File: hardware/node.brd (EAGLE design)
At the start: 16.5 x 25.7 mm, 56 parts, among them IC1 MAX1555, Q1 P-MOSFET, U1 ATMEGA32U4, U2 MCP1703CB/TOREX-XC6206, Y1 8MHz

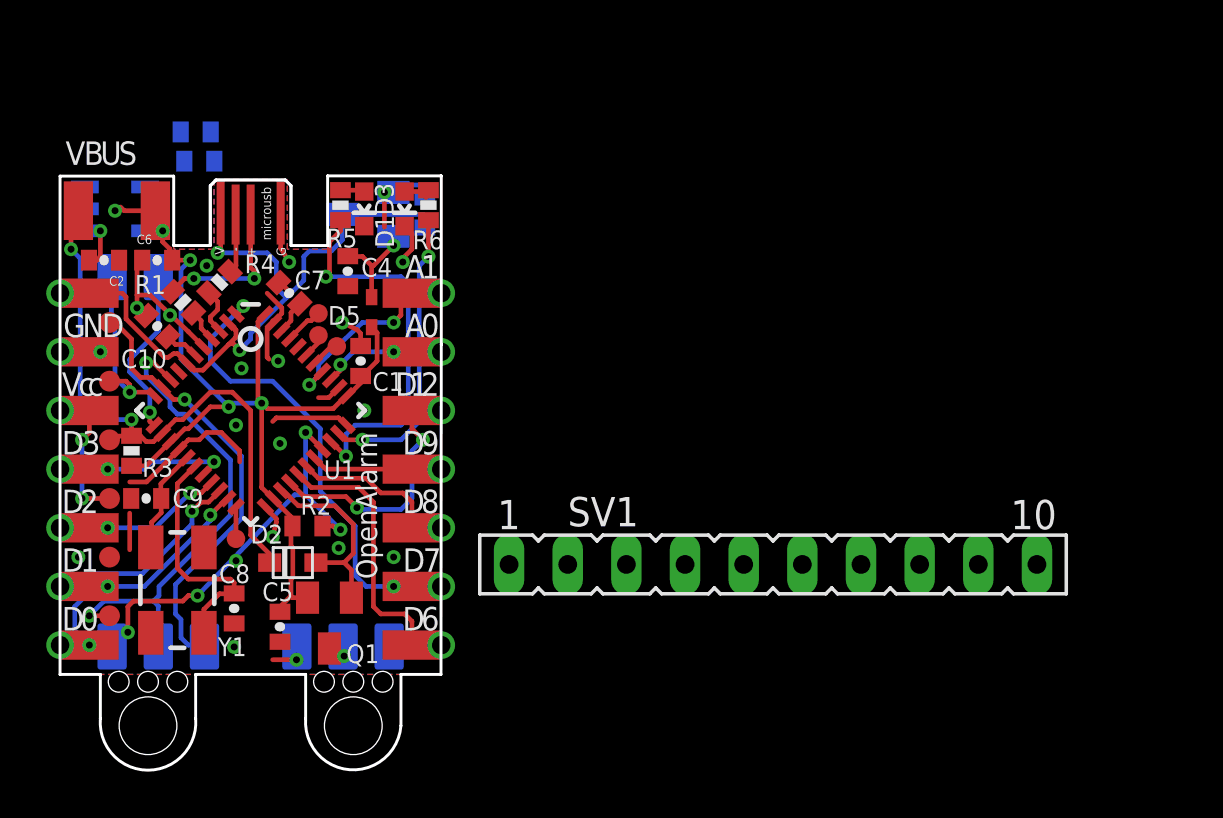
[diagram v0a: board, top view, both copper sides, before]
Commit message: New node
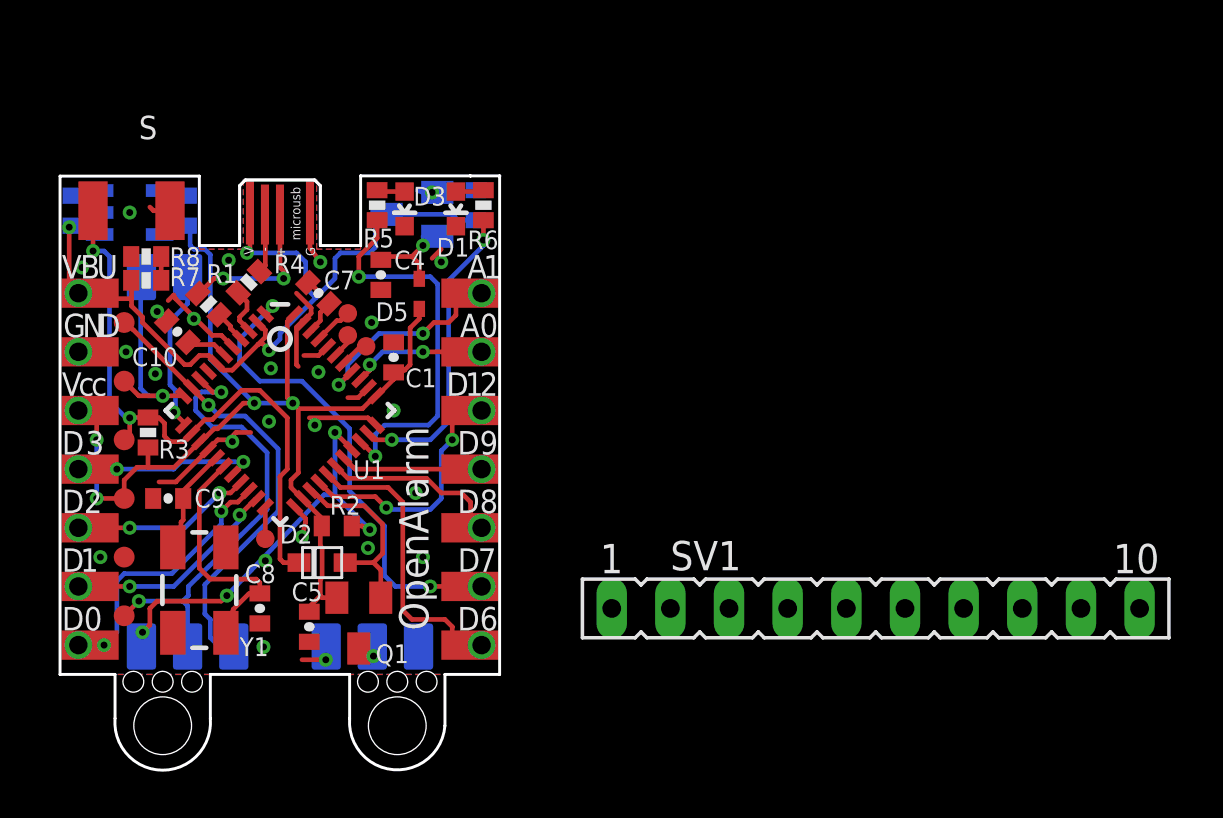
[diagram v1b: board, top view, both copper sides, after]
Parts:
- moved R8 5.81 mm to (3.73, 18.1), flipped to the top
- moved R7 5.65 mm to (3.73, 17.1), flipped to the top, turned to 180 degrees
- moved SV1 4.84 mm to (35.3, 2.86)
- moved PAD1 2.54 mm to (17.8, 8.89)
- moved PAD11 2.54 mm to (17.8, 6.35)
- moved PAD2 2.54 mm to (17.8, 3.81)
- moved PAD3 2.54 mm to (17.8, 11.4)
- moved PAD4 2.54 mm to (17.8, 1.27)
- moved PAD5 2.54 mm to (17.8, 16.5)
- moved PAD6 2.54 mm to (17.8, 14.0)
- moved C2 2.53 mm to (0.56, 20.1), flipped to the bottom, turned to 270 degrees
- moved C6 2.49 mm to (5.48, 20.1), flipped to the bottom, turned to 270 degrees
- moved R6 2.38 mm to (18.3, 20.3)
- moved C3 2.25 mm to (18.0, 20.3)
- moved D1 2.22 mm to (17.1, 20.2)
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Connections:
- removed net N$9: C2.2, IC1.1
- net VBUS: now also C2.2, IC1.1
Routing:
- net GND: track 35.2 -> 24.7 mm, vias 21 -> 25
- net VBUS: track 29.5 -> 37.0 mm, vias 2 -> 3
- net VCC: track 45.2 -> 50.3 mm, vias 6 -> 4
- net N$9: track 2.33 -> 0.00 mm, vias 1 -> 0
- net A4: track 0.01 -> 2.21 mm
- net D6: track 11.3 -> 12.6 mm
- net A1: track 7.72 -> 9.01 mm
- net D9: track 4.43 -> 5.70 mm
- net D7: track 19.1 -> 20.4 mm
- net D3: track 6.26 -> 7.53 mm
- net D2: track 6.11 -> 7.38 mm
- net D1: track 7.73 -> 9.00 mm
- net A0: track 4.21 -> 5.48 mm
- net D8: track 6.34 -> 7.61 mm
- net RESET: track 26.0 -> 27.2 mm
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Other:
- board size 16.5 x 25.7 mm -> 19.1 x 25.7 mm

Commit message: Node
Avancement
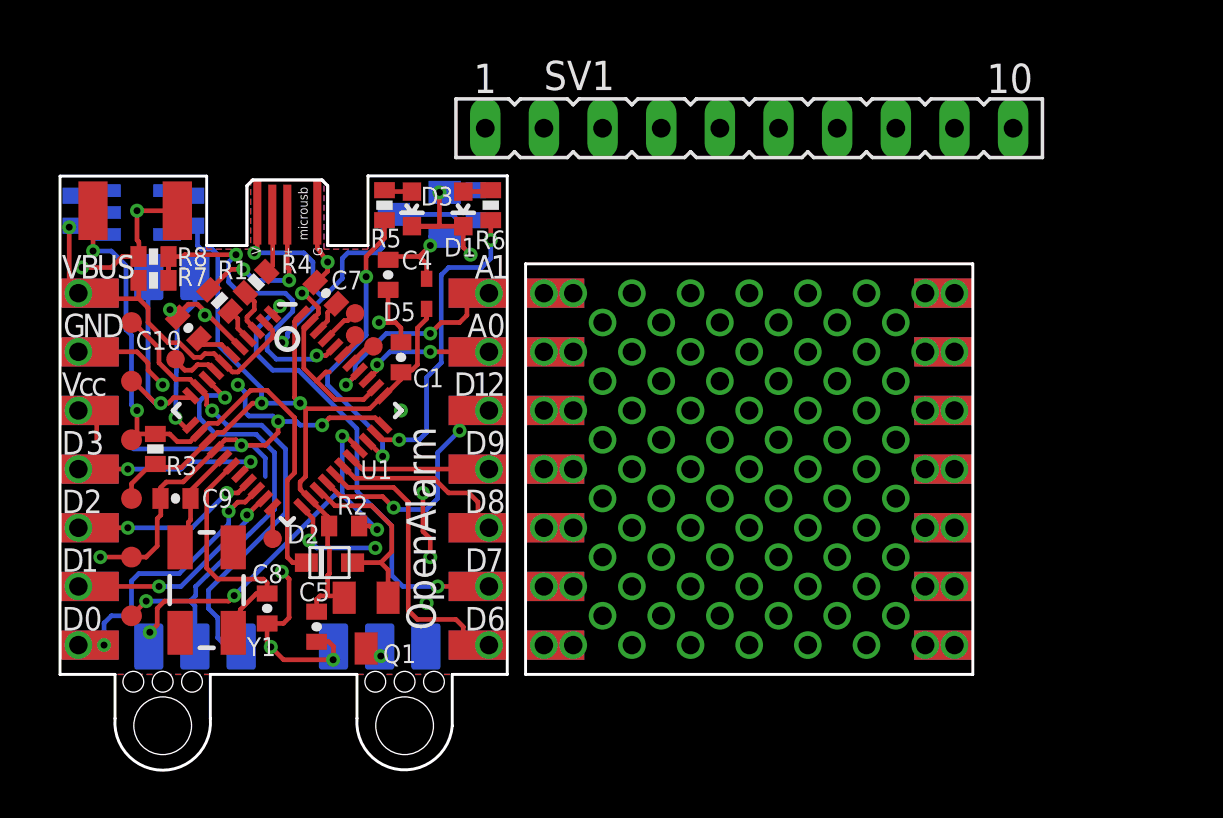
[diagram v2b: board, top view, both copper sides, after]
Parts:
- added PAD17, PAD18, PAD19, PAD20, PAD21, PAD22, PAD23, PAD24, PAD25, PAD26, PAD27, PAD28, PAD29, PAD30, PAD31, PAD32, PAD33, PAD34, PAD35, PAD36, PAD37, PAD38, PAD39, PAD40, PAD41, PAD42, PAD43, PAD44, PAD45, PAD46, PAD47, PAD48, PAD49, PAD50, PAD51, PAD52, PAD53, PAD54, PAD55, PAD56, PAD57, PAD58: (no value), wirepad:SMD1,27-2,54
- added TP11: TPTP08R, testpad:TP08R
- moved SV1 21.5 mm to (29.8, 23.7)
- moved R3 0.78 mm to (4.13, 9.76)
- moved C10 0.50 mm to (5.56, 15.0)
- moved R1 0.50 mm to (6.91, 16.2)
- moved C1 0.32 mm to (14.8, 13.7)
- moved C4 0.32 mm to (14.2, 17.3)
- moved C5 0.32 mm to (11.1, 2.06)
- moved C7 0.32 mm to (11.5, 16.5)
- moved D3 0.32 mm to (15.2, 20.2)
- moved D5 0.32 mm to (15.9, 16.4)
- moved Q1 0.32 mm to (13.3, 2.22)
- moved TP10 0.32 mm to (12.8, 15.6)
- moved TP8 0.32 mm to (12.8, 14.7)
- moved IC1 0.32 mm to (3.33, 20.0)
- moved C6 0.32 mm to (5.79, 20.1)
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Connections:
- net TXLED_NOTUSED renamed TXLED
- removed net RXLED_NOTUSED: U1.8
- new net N$13: PAD33.1, PAD34.1
- new net N$27: PAD35.1, PAD36.1
- new net N$29: PAD37.1, PAD38.1
- new net N$30: PAD39.1, PAD40.1
- new net N$31: PAD41.1, PAD42.1
- new net N$32: PAD43.1, PAD44.1
- new net N$40: PAD45.1, PAD46.1
- new net N$41: PAD47.1, PAD48.1
- new net N$42: PAD49.1, PAD50.1
- new net N$43: PAD51.1, PAD52.1
- new net N$44: PAD53.1, PAD54.1
- new net N$45: PAD55.1, PAD56.1
- new net N$46: PAD57.1, PAD58.1
- new net N$9: PAD31.1, PAD32.1
- new net RXLED: TP11.TP, U1.8
- net A0: now also PAD29.1
- net A1: now also PAD30.1
- net D0: now also PAD23.1
- net D1: now also PAD22.1
- net D12: now also PAD28.1
- net D2: now also PAD21.1
- net D3: now also PAD20.1
- net D6: now also PAD24.1
- net D7: now also PAD25.1
- net D8: now also PAD26.1
- net D9: now also PAD27.1
- net GND: now also PAD18.1
- net VBUS: now also PAD17.1
- net VCC: now also PAD19.1
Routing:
- net GND: track 24.7 -> 80.1 mm, vias 25 -> 24
- net A4: track 2.21 -> 15.5 mm, vias 0 -> 2
- net VCC: track 50.3 -> 46.1 mm, vias 4 -> 2
- net D5_LED_GREEN: track 17.0 -> 13.2 mm
- net RXLED: track 0.00 -> 2.19 mm
- net D7: track 20.4 -> 19.6 mm
- net MOSI: track 19.9 -> 20.7 mm
- net D6: track 12.6 -> 13.2 mm
- net D+: track 6.94 -> 7.45 mm
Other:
- board size 19.1 x 25.7 mm -> 39.5 x 25.7 mm
- board text removed: "INT: D0, D1, D2, D3, D7"
- board text removed: "PCINT: D8, D9"
